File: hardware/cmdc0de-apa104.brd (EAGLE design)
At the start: 101.6 x 74.6 mm, 128 parts, among them IC1 ATTINY13A-SSU, J1 1x8 header

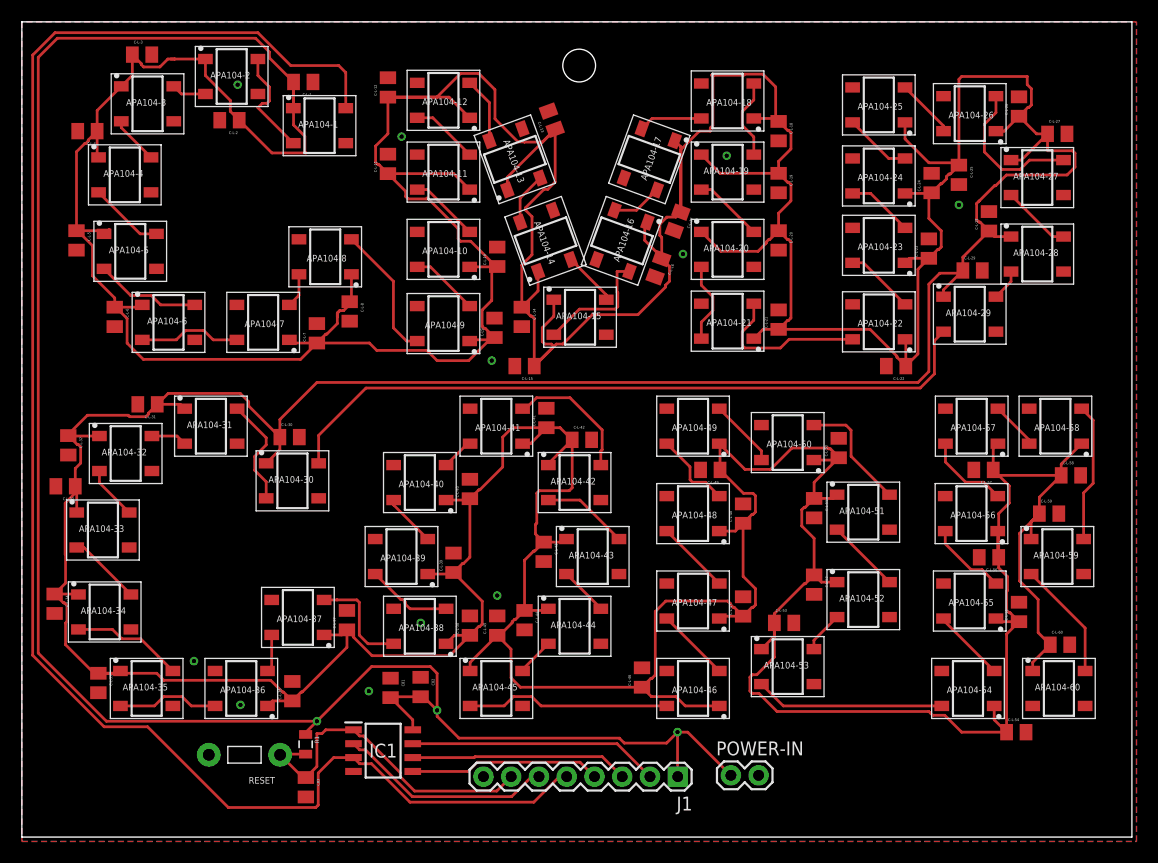
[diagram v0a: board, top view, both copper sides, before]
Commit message: fixed wire pieces
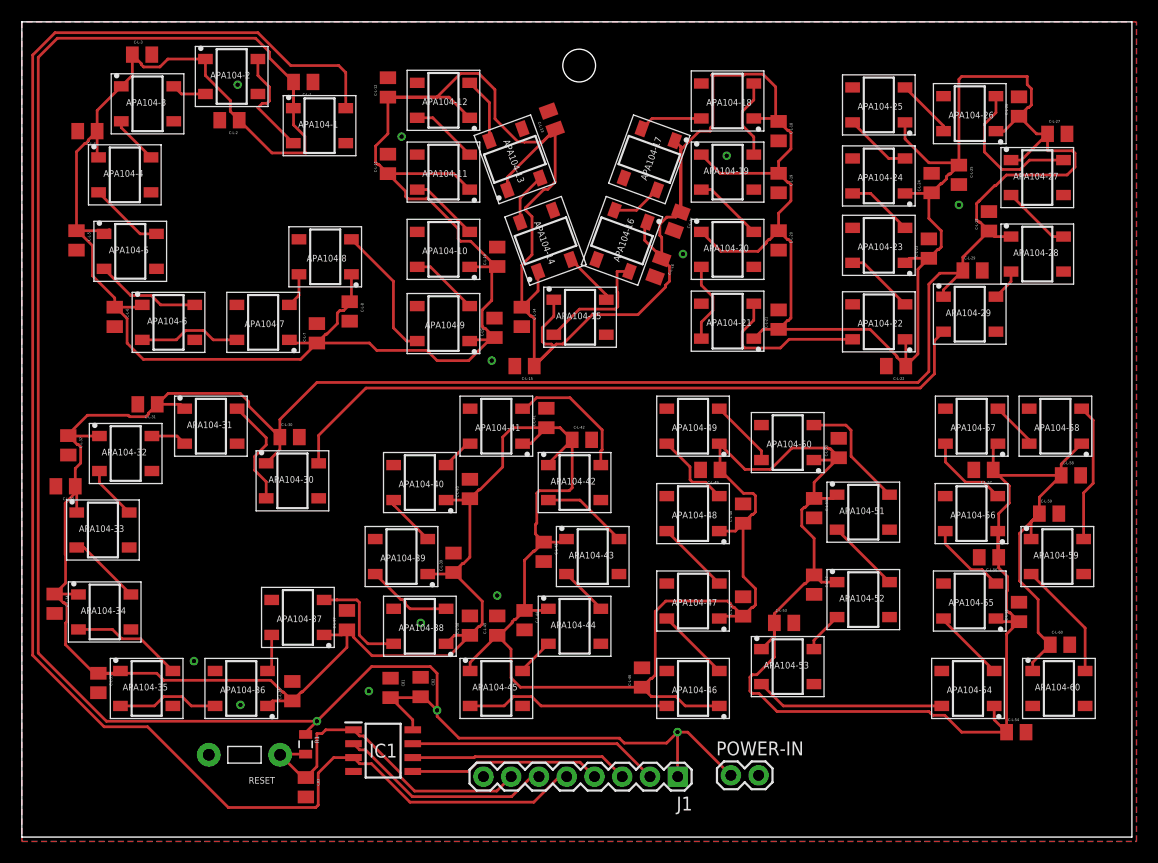
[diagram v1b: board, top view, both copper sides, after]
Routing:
- net VDD: track 1082.9 -> 1079.3 mm
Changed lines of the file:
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@@
 <contactref element="C-L-59" pad="1"/>
 <contactref element="C-L-60" pad="1"/>
-<wire x1="16.8" y1="96.6" x2="14" y2="96.6" width="0.254" layer="1"/>
-<wire x1="14" y1="96.6" x2="13.6" y2="96.6" width="0.254" layer="1"/>
-<wire x1="9.1" y1="94.1" x2="9" y2="94" width="0.254" layer="1"/>
+<wire x1="16.8" y1="96.6" x2="13.3613125" y2="96.6" width="0.254" layer="1"/>
 <wire x1="6.8636" y1="87.7564" x2="7.02" y2="87.6" width="0.254" layer="1"/>
-<wire x1="10.7836" y1="73.8636" x2="11.02" y2="74.1" width="0.254" layer="1"/>
-<wire x1="24.7436" y1="70.6364" x2="24.69" y2="70.69" width="0.254" layer="1"/>
-<wire x1="24.69" y1="70.69" x2="24.48" y2="70.9" width="0.254" layer="1"/>
-<wire x1="24.7436" y1="70.6364" x2="24.69" y2="70.69" width="0.254" layer="1"/>
-<wire x1="24.69" y1="70.69" x2="24.48" y2="70.9" width="0.254" layer="1"/>
+<wire x1="24.769" y1="70.611" x2="24.48" y2="70.9" width="0.254" layer="1"/>
 <contactref element="IC1" pad="8"/>
 <contactref element="C81" pad="2"/>
@@
 <wire x1="12.6310125" y1="95.8697" x2="11.1469875" y2="95.8697" width="0.254" layer="1"/>
 <wire x1="11.1469875" y1="95.8697" x2="10.9238" y2="96.0928875" width="0.254" layer="1"/>
-<wire x1="14" y1="96.6" x2="13.3613125" y2="96.6" width="0.254" layer="1"/>
 <wire x1="10.9238" y1="96.0928875" x2="10.9238" y2="96.1872" width="0.254" layer="1"/>
 <wire x1="13.3613125" y1="96.6" x2="12.6310125" y2="95.8697" width="0.254" layer="1"/>
 <wire x1="10.9238" y1="96.1872" x2="10.111" y2="97" width="0.254" layer="1"/>
 <wire x1="10.111" y1="97" x2="10.111" y2="95.111" width="0.254" layer="1"/>
-<wire x1="10.111" y1="95.111" x2="9" y2="94" width="0.254" layer="1"/>
+<wire x1="10.111" y1="95.111" x2="9.1" y2="94.1" width="0.254" layer="1"/>
 <wire x1="27" y1="70.611" x2="31.800875" y2="70.611" width="0.254" layer="1"/>
 <wire x1="37.066" y1="69.934" x2="38" y2="69" width="0.254" layer="1"/>
@@
 <wire x1="32.477875" y1="69.934" x2="37.066" y2="69.934" width="0.254" layer="1"/>
 <wire x1="38" y1="69" x2="40.889" y2="69" width="0.254" layer="1"/>
-<wire x1="41.301" y1="71.111" x2="41.095" y2="70.905" width="0.254" layer="1"/>
 <wire x1="41.095" y1="70.905" x2="40.98" y2="70.79" width="0.254" layer="1"/>
 <wire x1="43.5" y1="77.611" x2="43.469" y2="77.58" width="0.254" layer="1"/>
@@
 <wire x1="46" y1="89" x2="47.639440625" y2="89" width="0.254" layer="1"/>
 <wire x1="47.639440625" y1="89" x2="48.804053125" y2="90.1646125" width="0.254" layer="1"/>
-<wire x1="48.804053125" y1="90.1646125" x2="49" y2="89.968665625" width="0.254" layer="1"/>
 <wire x1="44.617503125" y1="84.617503125" x2="44.4273375" y2="84.617503125" width="0.254" layer="1"/>
-<wire x1="46.5" y1="68.889" x2="46.6945" y2="68.6945" width="0.254" layer="1"/>
-<wire x1="46.6945" y1="68.6945" x2="46.889" y2="68.5" width="0.254" layer="1"/>
+<wire x1="46.5" y1="68.889" x2="46.889" y2="68.5" width="0.254" layer="1"/>
 <wire x1="48.804053125" y1="90.1646125" x2="44.4273375" y2="85.787896875" width="0.254" layer="1"/>
 <wire x1="44.4273375" y1="85.787896875" x2="44.4273375" y2="84.617503125" width="0.254" layer="1"/>
@@
 <wire x1="42.1197" y1="73.6310125" x2="43" y2="74.5113125" width="0.254" layer="1"/>
 <wire x1="43.25" y1="71.111" x2="42.4372" y2="71.9238" width="0.254" layer="1"/>
-<wire x1="58.216003125" y1="77.997334375" x2="58.554053125" y2="78.335384375" width="0.254" layer="1"/>
 <wire x1="58.554053125" y1="78.335384375" x2="58.554053125" y2="78.445946875" width="0.254" layer="1"/>
 <wire x1="58.554053125" y1="78.445946875" x2="57" y2="80" width="0.254" layer="1"/>
@@
 <wire x1="6.889" y1="87.7818" x2="6.8636" y2="87.7564" width="0.254" layer="1"/>
 <wire x1="6.889" y1="90" x2="6.889" y2="91.889" width="0.254" layer="1"/>
-<wire x1="6.889" y1="91.889" x2="9" y2="94" width="0.254" layer="1"/>
+<wire x1="6.889" y1="91.889" x2="9.1" y2="94.1" width="0.254" layer="1"/>
 <wire x1="8.5" y1="74.7311875" x2="8.5" y2="73.889" width="0.254" layer="1"/>
 <wire x1="6.464" y1="76.7671875" x2="8.5" y2="74.7311875" width="0.254" layer="1"/>
 <wire x1="6.464" y1="76.7671875" x2="6.464" y2="79.5193125" width="0.254" layer="1"/>
 <wire x1="8.5" y1="73.889" x2="9" y2="73.889" width="0.254" layer="1"/>
-<wire x1="9" y1="73.889" x2="10.809" y2="73.889" width="0.254" layer="1"/>
-<wire x1="10.809" y1="73.889" x2="11.02" y2="74.1" width="0.254" layer="1"/>
 <wire x1="11.11559375" y1="69.11559375" x2="9.6303" y2="70.6008875" width="0.254" layer="1"/>
 <wire x1="9" y1="73.4833125" x2="9" y2="73.889" width="0.254" layer="1"/>
@@
 <wire x1="9.6303" y1="72.8530125" x2="9" y2="73.4833125" width="0.254" layer="1"/>
 <wire x1="27" y1="70.611" x2="24.769" y2="70.611" width="0.254" layer="1"/>
-<wire x1="24.769" y1="70.611" x2="24.69" y2="70.69" width="0.254" layer="1"/>
 <wire x1="27" y1="70.611" x2="27.8128" y2="71.4238" width="0.254" layer="1"/>
 <wire x1="27.8128" y1="71.4238" x2="27.9071125" y2="71.4238" width="0.254" layer="1"/>
-<wire x1="28.8697" y1="73.3530125" x2="29.0928875" y2="73.5762" width="0.254" layer="1"/>
 <wire x1="27.9071125" y1="71.4238" x2="28.8697" y2="72.3863875" width="0.254" layer="1"/>
-<wire x1="28.8697" y1="72.3863875" x2="28.8697" y2="73" width="0.254" layer="1"/>
-<wire x1="28.8697" y1="73" x2="28.8697" y2="73.3530125" width="0.254" layer="1"/>
+<wire x1="28.8697" y1="72.3863875" x2="28.8697" y2="73.3530125" width="0.254" layer="1"/>
 <wire x1="46.889" y1="68.5" x2="48.903" y2="70.514" width="0.254" layer="1"/>
 <wire x1="48.903" y1="70.514" x2="49.5128125" y2="70.514" width="0.254" layer="1"/>
@@
 <wire x1="12.389" y1="65" x2="14.5" y2="65" width="0.254" layer="1"/>
 <wire x1="14.5" y1="65" x2="14.9" y2="64.6" width="0.254" layer="1"/>
-<wire x1="4.25" y1="62.25" x2="4.25" y2="62.139" width="0.254" layer="1"/>
-<wire x1="4.25" y1="62.139" x2="4.461" y2="62.35" width="0.254" layer="1"/>
 <wire x1="3" y1="47.639" x2="5.141" y2="47.639" width="0.254" layer="1"/>
 <wire x1="5.141" y1="47.639" x2="5.18" y2="47.6" width="0.254" layer="1"/>
@@
 <wire x1="94.111" y1="43" x2="92.5" y2="41.389" width="0.254" layer="1"/>
 <wire x1="92.5" y1="41.389" x2="92.5" y2="40.6" width="0.254" layer="1"/>
-<wire x1="37.009" y1="38.241" x2="37" y2="38.241" width="0.254" layer="1"/>
 <wire x1="37" y1="38.241" x2="36.49" y2="38.241" width="0.254" layer="1"/>
-<wire x1="33.91" y1="37.991" x2="33.74" y2="38.161" width="0.254" layer="1"/>
-<wire x1="33.74" y1="38.161" x2="33.9505" y2="37.9505" width="0.254" layer="1"/>
 <contactref element="J1" pad="1"/>
-<wire x1="33.9505" y1="37.9505" x2="34.022" y2="37.879" width="0.254" layer="1"/>
 <contactref element="R1" pad="1"/>
 <via x="27" y="36" extent="1-16" drill="0.4"/>
-<wire x1="36.49" y1="38.241" x2="34.241" y2="38.241" width="0.254" layer="1"/>
-<wire x1="34.241" y1="38.241" x2="33.9505" y2="37.9505" width="0.254" layer="1"/>
-<wire x1="33.74" y1="38.161" x2="35.772" y2="36.129" width="0.254" layer="1"/>
-<wire x1="35.772" y1="36.129" x2="35.772" y2="35.215" width="0.254" layer="1"/>
 <via x="38" y="37" extent="1-16" drill="0.4"/>
 <via x="60" y="35" extent="1-16" drill="0.4"/>
@@
 <wire x1="49.559" y1="52.389" x2="49.84" y2="52.67" width="0.254" layer="1"/>
 <wire x1="7.52" y1="80.6" x2="7.6" y2="80.6" width="0.254" layer="1"/>
-<wire x1="7.6" y1="80.6" x2="8" y2="81" width="0.254" layer="1"/>
+<wire x1="7.6" y1="80.6" x2="7.889" y2="80.889" width="0.254" layer="1"/>
 <wire x1="8" y1="81" x2="7.889" y2="80.889" width="0.254" layer="1"/>
 <wire x1="7.889" y1="80.889" x2="5" y2="80.889" width="0.254" layer="1"/>
 <wire x1="30" y1="74.1303" x2="30" y2="74.389" width="0.254" layer="1"/>
-<wire x1="28.8697" y1="73" x2="28.8697" y2="73.3530125" width="0.254" layer="1"/>
 <wire x1="28.8697" y1="73.3530125" x2="29.0928875" y2="73.5762" width="0.254" layer="1"/>
 <wire x1="29.0928875" y1="73.5762" x2="29.4459" y2="73.5762" width="0.254" layer="1"/>
@@
 <wire x1="40" y1="34.453" x2="38" y2="36.453" width="0.254" layer="1"/>
 <wire x1="38" y1="36.453" x2="38" y2="37" width="0.254" layer="1"/>
+<wire x1="8.5" y1="73.889" x2="10.809" y2="73.889" width="0.254" layer="1"/>
+<wire x1="10.809" y1="73.889" x2="11.02" y2="74.1" width="0.254" layer="1"/>
+<wire x1="36.49" y1="38.241" x2="36.41" y2="38.161" width="0.254" layer="1"/>
+<wire x1="36.41" y1="38.161" x2="33.74" y2="38.161" width="0.254" layer="1"/>
+<wire x1="33.74" y1="38.161" x2="35.772" y2="36.129" width="0.254" layer="1"/>
+<wire x1="35.772" y1="36.129" x2="35.772" y2="35.215" width="0.254" layer="1"/>
 </signal>
 <signal name="GPIO_APA104_DATA1">

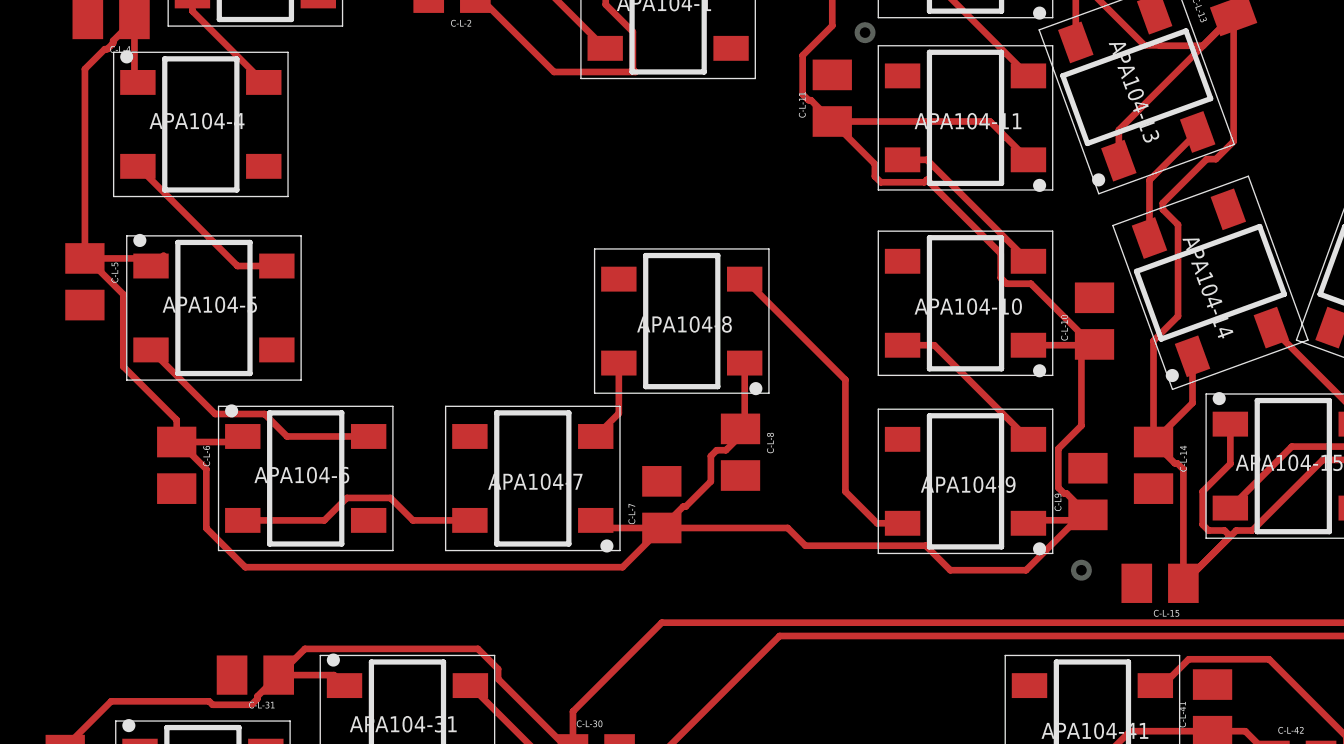
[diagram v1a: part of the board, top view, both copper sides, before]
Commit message: board and gerbers
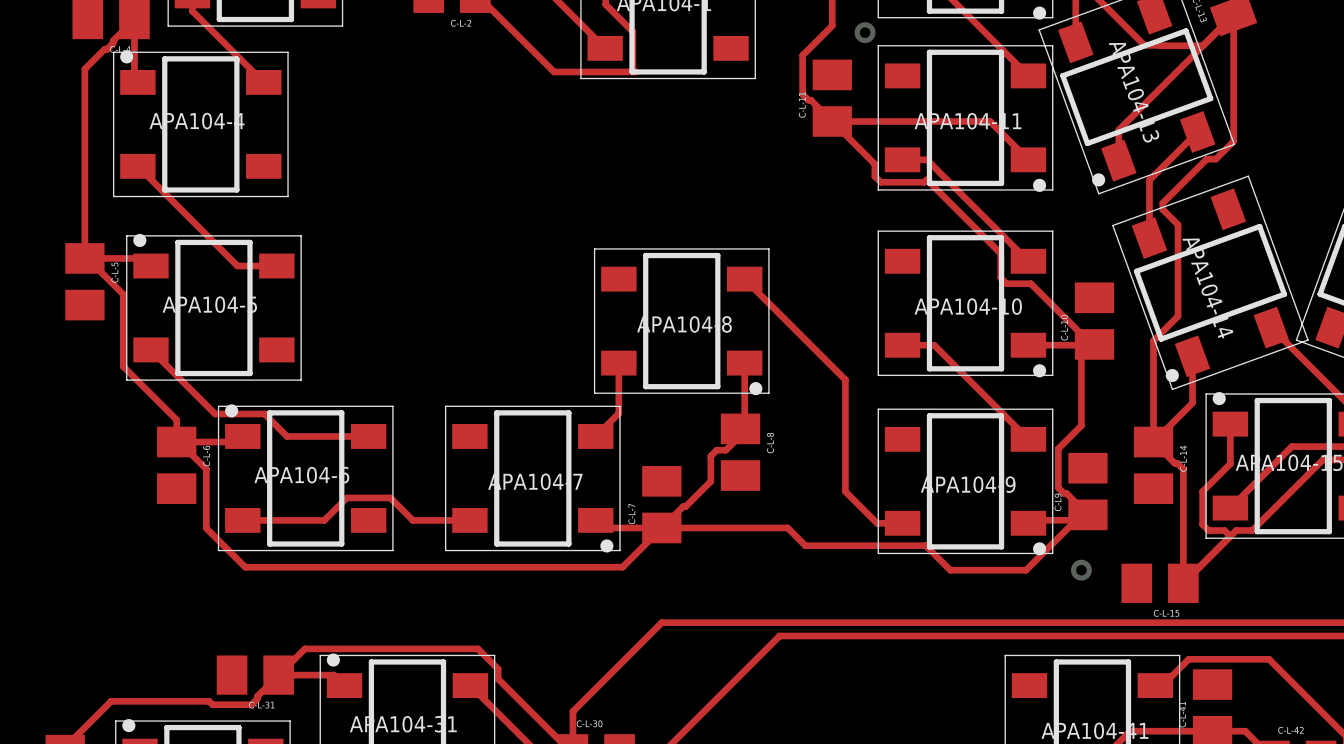
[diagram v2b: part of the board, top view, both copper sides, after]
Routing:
- net VDD: track 1079.3 -> 1078.4 mm
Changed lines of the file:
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@@
 <wire x1="46" y1="89" x2="47.639440625" y2="89" width="0.254" layer="1"/>
 <wire x1="47.639440625" y1="89" x2="48.804053125" y2="90.1646125" width="0.254" layer="1"/>
-<wire x1="44.617503125" y1="84.617503125" x2="44.4273375" y2="84.617503125" width="0.254" layer="1"/>
-<wire x1="46.5" y1="68.889" x2="46.889" y2="68.5" width="0.254" layer="1"/>
 <wire x1="48.804053125" y1="90.1646125" x2="44.4273375" y2="85.787896875" width="0.254" layer="1"/>
 <wire x1="44.4273375" y1="85.787896875" x2="44.4273375" y2="84.617503125" width="0.254" layer="1"/>
@@
 <wire x1="7.52" y1="80.6" x2="7.6" y2="80.6" width="0.254" layer="1"/>
 <wire x1="7.6" y1="80.6" x2="7.889" y2="80.889" width="0.254" layer="1"/>
-<wire x1="8" y1="81" x2="7.889" y2="80.889" width="0.254" layer="1"/>
 <wire x1="7.889" y1="80.889" x2="5" y2="80.889" width="0.254" layer="1"/>
 <wire x1="30" y1="74.1303" x2="30" y2="74.389" width="0.254" layer="1"/>
